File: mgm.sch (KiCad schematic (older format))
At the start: 35 parts, among them J13 0826-1X1T-GH-F, J18 DF40HC_3.0_-100DS-0.4V_51_PNP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, J19 DF40HC_3.0_-100DS-0.4V_51_PNP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, M1 Fan_4pin, M2 Fan_4pin, M3 Fan_4pin, Q1 2N7002K, U10 rpi_cm4

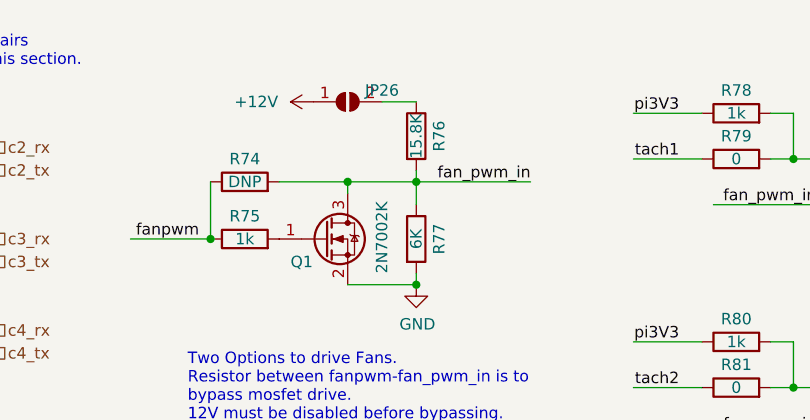
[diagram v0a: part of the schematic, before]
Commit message: DFM
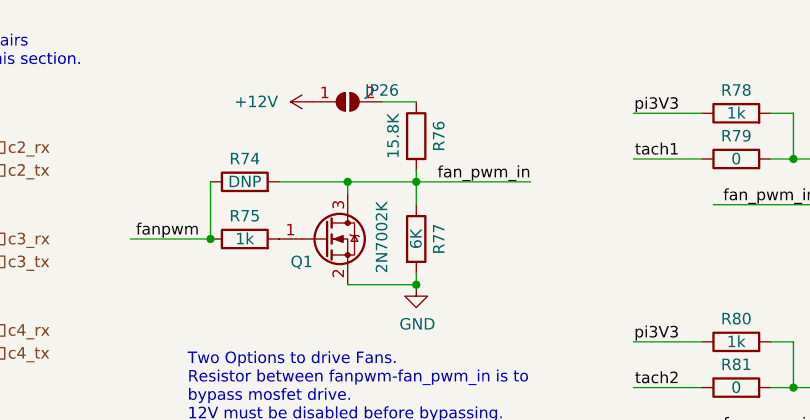
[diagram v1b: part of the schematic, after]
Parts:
- C81: JLC# (none) -> C312983
- C82, C83, C84: JLC# (none) -> C15850
- C86, C88: JLC# (none) -> C1525
- J18, J19: JLC# (none) -> C424649; LCSC# C424649 -> (none)
- Q1: JLC# (none) -> C504047
- R76: JLC# (none) -> C26956
- R79, R81, R83: JLC# (none) -> C17168
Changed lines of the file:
@@
 F 2 "Capacitor_SMD:C_0805_2012Metric" H 2338 7050 50  0001 C CNN
 F 3 "~" H 2300 7200 50  0001 C CNN
+F 4 "C15850" H 2300 7200 50  0001 C CNN "JLC#"
 	1    2300 7200
 	1    0    0    -1
@@
 F 2 "Capacitor_SMD:C_0805_2012Metric" H 2088 7050 50  0001 C CNN
 F 3 "~" H 2050 7200 50  0001 C CNN
+F 4 "C15850" H 2050 7200 50  0001 C CNN "JLC#"
 	1    2050 7200
 	1    0    0    -1
@@
 F 2 "Capacitor_SMD:C_0805_2012Metric" H 1838 7050 50  0001 C CNN
 F 3 "~" H 1800 7200 50  0001 C CNN
+F 4 "C15850" H 1800 7200 50  0001 C CNN "JLC#"
 	1    1800 7200
 	1    0    0    -1
@@
 F 2 "Capacitor_SMD:C_1206_3216Metric" H 1538 7050 50  0001 C CNN
 F 3 "~" H 1500 7200 50  0001 C CNN
+F 4 "C312983" H 1500 7200 50  0001 C CNN "JLC#"
 	1    1500 7200
 	1    0    0    -1
@@
 F 2 "Capacitor_SMD:C_0402_1005Metric" H 2888 7050 50  0001 C CNN
 F 3 "~" H 2850 7200 50  0001 C CNN
+F 4 "C1525" H 2850 7200 50  0001 C CNN "JLC#"
 	1    2850 7200
 	1    0    0    -1
@@
 F 2 "Capacitor_SMD:C_0402_1005Metric" H 8138 5000 50  0001 C CNN
 F 3 "~" H 8100 5150 50  0001 C CNN
+F 4 "C1525" H 8100 5150 50  0001 C CNN "JLC#"
 	1    8100 5150
 	-1   0    0    -1
@@
 F 2 "Resistor_SMD:R_0402_1005Metric" V 8730 1400 50  0001 C CNN
 F 3 "~" H 8800 1400 50  0001 C CNN
+F 4 "C17168" V 8800 1400 50  0001 C CNN "JLC#"
 	1    8800 1400
 	0    -1   -1   0
@@
 F 2 "Resistor_SMD:R_0402_1005Metric" V 8730 2400 50  0001 C CNN
 F 3 "~" H 8800 2400 50  0001 C CNN
+F 4 "C17168" V 8800 2400 50  0001 C CNN "JLC#"
 	1    8800 2400
 	0    -1   -1   0
@@
 F 2 "Package_TO_SOT_SMD:SOT-23" H 7200 1675 50  0001 L CIN
 F 3 "https://www.diodes.com/assets/Datasheets/ds30896.pdf" H 7000 1750 50  0001 L CNN
+F 4 "C504047" H 7000 1750 50  0001 C CNN "JLC#"
 	1    7000 1750
 	1    0    0    -1
@@
 AR Path="/613B5606/61B21EED" Ref="R76"  Part="1"
 F 0 "R76" V 7500 1300 50  0000 C CNN
-F 1 "15.8K" V 7400 1300 50  0000 C CNN
+F 1 "15.8K" V 7300 1300 50  0000 C CNN
 F 2 "Resistor_SMD:R_0402_1005Metric" V 7330 1300 50  0001 C CNN
 F 3 "~" H 7400 1300 50  0001 C CNN
+F 4 "C26956" V 7400 1300 50  0001 C CNN "JLC#"
 	1    7400 1300
 	1    0    0    -1
@@
 F 2 "Resistor_SMD:R_0402_1005Metric" V 6780 3150 50  0001 C CNN
 F 3 "~" H 6850 3150 50  0001 C CNN
+F 4 "C17168" V 6850 3150 50  0001 C CNN "JLC#"
 	1    6850 3150
 	0    -1   -1   0
@@
 F 10 "DF40HC(3.0)-100DS-0.4V(51" H 5200 6650 50  0001 L CNN "Arrow Part Number"
 F 11 "https://www.arrow.com/en/products/df40hc-3.0-100ds-0.4v-51/hirose-electric" H 5200 6550 50  0001 L CNN "Arrow Price/Stock"
-F 12 "C424649" H 4628 7259 50  0000 L CNN "LCSC#"
+F 12 "C424649" H 4628 7259 50  0000 L CNN "JLC#"
 	1    4350 7350
 	1    0    0    -1
@@
 F 10 "DF40HC(3.0)-100DS-0.4V(51" H 5200 6200 50  0001 L CNN "Arrow Part Number"
 F 11 "https://www.arrow.com/en/products/df40hc-3.0-100ds-0.4v-51/hirose-electric" H 5200 6100 50  0001 L CNN "Arrow Price/Stock"
-F 12 "C424649" H 4628 6809 50  0000 L CNN "LCSC#"
+F 12 "C424649" H 4628 6809 50  0000 L CNN "JLC#"
 	1    4350 6900
 	1    0    0    -1
